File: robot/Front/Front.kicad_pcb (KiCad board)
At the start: 2 copper layers, 40 x 40 mm, 42 parts, among them J1 USB_B_Micro, Q1 BC849, Q2 BC849, SW2 SW_Push, U1 CH340C, U10 ESP32-WROOM-32, U2 CJVL53L0XV2, U3 LD1117S33CTR

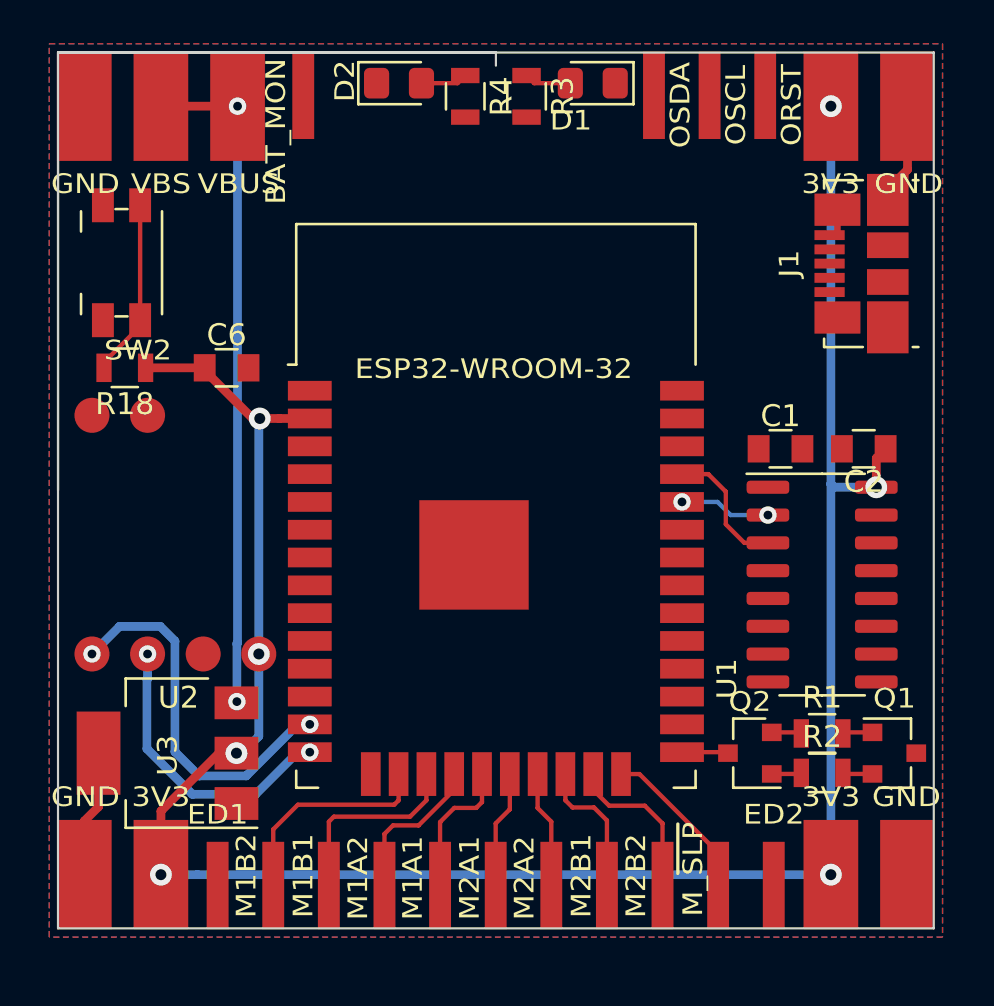
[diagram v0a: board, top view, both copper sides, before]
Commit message: Finish Front redesign
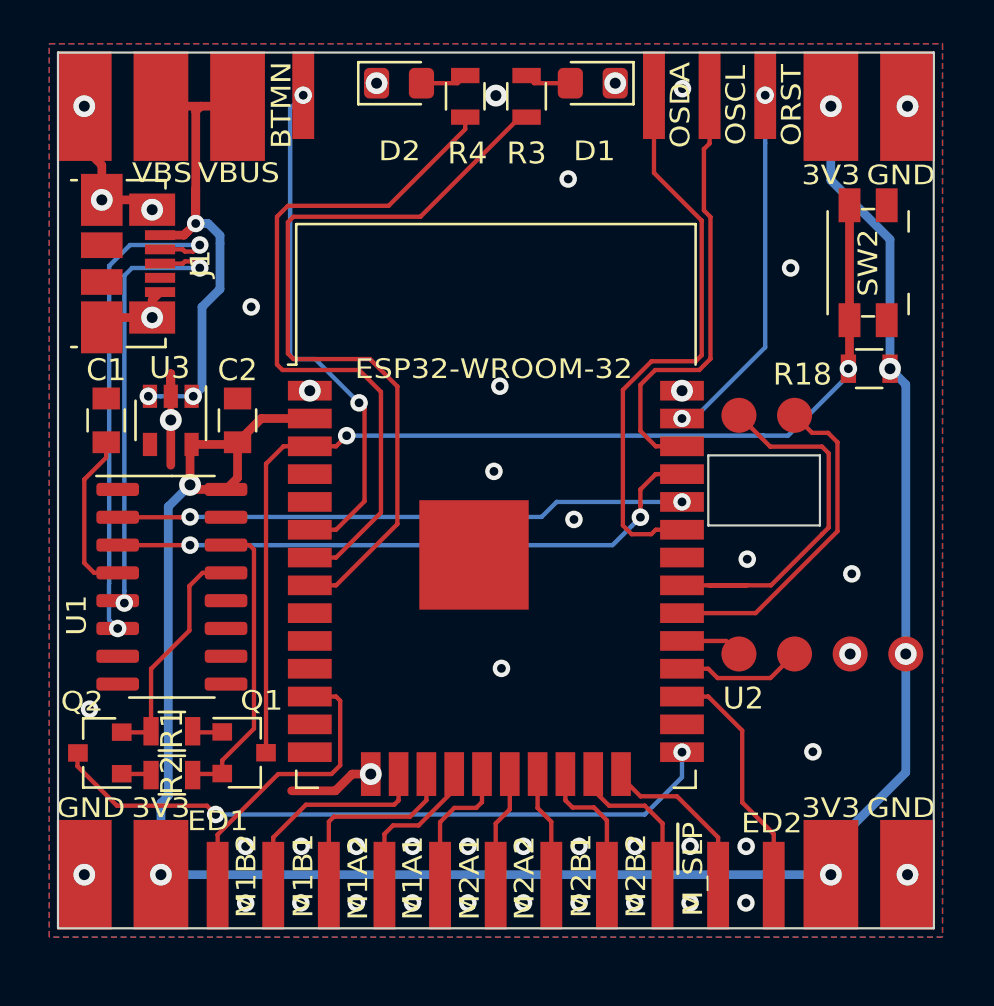
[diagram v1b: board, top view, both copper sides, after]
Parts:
- removed C6: 10µ, Capacitors_SMD:C_0805
- C2: value 10µ -> 22µ
- H11: value BAT_MON -> BTMN
- U3: value LD1117S33CTR -> SPX3819M5-L-3-3; footprint Package_TO_SOT_SMD:SOT-223 -> Package_TO_SOT_SMD:SOT-23-5
- moved J1 35.9 mm to (197.5, 112.6), turned to 270 degrees
- moved SW2 34.1 mm to (232.5, 112.6), turned to 270 degrees
- moved R18 34.0 mm to (232.6, 117.4)
- moved C1 30.8 mm to (197.7, 119.8), turned to 90 degrees
- moved R1 29.7 mm to (200.7, 134.0)
- moved R2 29.7 mm to (200.7, 136.0)
- moved U1 29.7 mm to (200.7, 127.4)
- moved Q1 29.7 mm to (204.0, 135.0)
- moved Q2 29.7 mm to (197.4, 135.0)
- moved U2 29.6 mm to (234.2, 129.9)
- moved C2 28.6 mm to (203.7, 119.8), turned to 90 degrees
- moved U3 15.2 mm to (200.7, 119.8), turned to 270 degrees
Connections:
- U10 pad 10: /BAT_MON -> (no net)
- U10 pad 12: (no net) -> /ED_IN1
- U10 pad 13: /OD_SDA -> (no net)
- U10 pad 14: /OD_SCL -> (no net)
- U10 pad 27: (no net) -> /ED_IN2
- U10 pad 28: (no net) -> /OD_SCL
- U10 pad 29: (no net) -> /OD_SDA
- U10 pad 30: /STATUS_LED_BLUE -> /OD_SHUT
- U10 pad 31: /STATUS_LED_GRN -> /OD_INTERRUPT
- U10 pad 6: /ED_IN1 -> /BAT_MON
- U10 pad 7: /ED_IN2 -> /STATUS_LED_GRN
- U10 pad 8: /OD_INTERRUPT -> /STATUS_LED_BLUE
- U10 pad 9: /OD_SHUT -> (no net)
- U3 pad 1: GND -> VBUS
- U3 pad 2: +3V3 -> GND
- U3 pad 4: GND -> (no net)
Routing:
- net /~RST: track 8.11 -> 49.8 mm, vias 0 -> 2
- net /STATUS_LED_BLUE: track 0.00 -> 36.0 mm
- net /STATUS_LED_GRN: track 0.00 -> 32.4 mm
- net /GPIO0: track 2.12 -> 31.0 mm, vias 0 -> 2
- net /OLED_SDA: track 0.00 -> 26.2 mm
- net /BAT_MON: track 0.00 -> 23.8 mm, vias 0 -> 2
- net /D-: track 0.00 -> 23.2 mm, vias 0 -> 2
- net /TXD-RXD: track 4.17 -> 26.6 mm
- net /RXD-TXD: track 6.10 -> 27.9 mm, vias 0 -> 2
- net /D+: track 0.00 -> 20.5 mm, vias 0 -> 2
- net /OLED_SCL: track 0.00 -> 20.3 mm
- net /OD_INTERRUPT: track 0.00 -> 17.7 mm
- net /OLED_~RES: track 0.00 -> 16.7 mm, vias 0 -> 2
- net /OD_SHUT: track 0.00 -> 15.2 mm
- net /ED_IN1: track 0.00 -> 15.2 mm
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- added copper zone on B.Cu, net GND
- removed copper zone on B.Cu, net (none)
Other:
- outline, holes or cut-outs redrawn
